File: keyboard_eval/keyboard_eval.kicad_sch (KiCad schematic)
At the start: 65 parts, among them IC1 IS31FL3733B-TQLS4, J1 Conn_01x03, J2 Conn_01x04, J3 Conn_01x04, J4 Conn_01x07, J5 Conn_01x03, J6 Conn_01x03, J7 Conn_01x06, SW1 RotaryEncoder_Switch

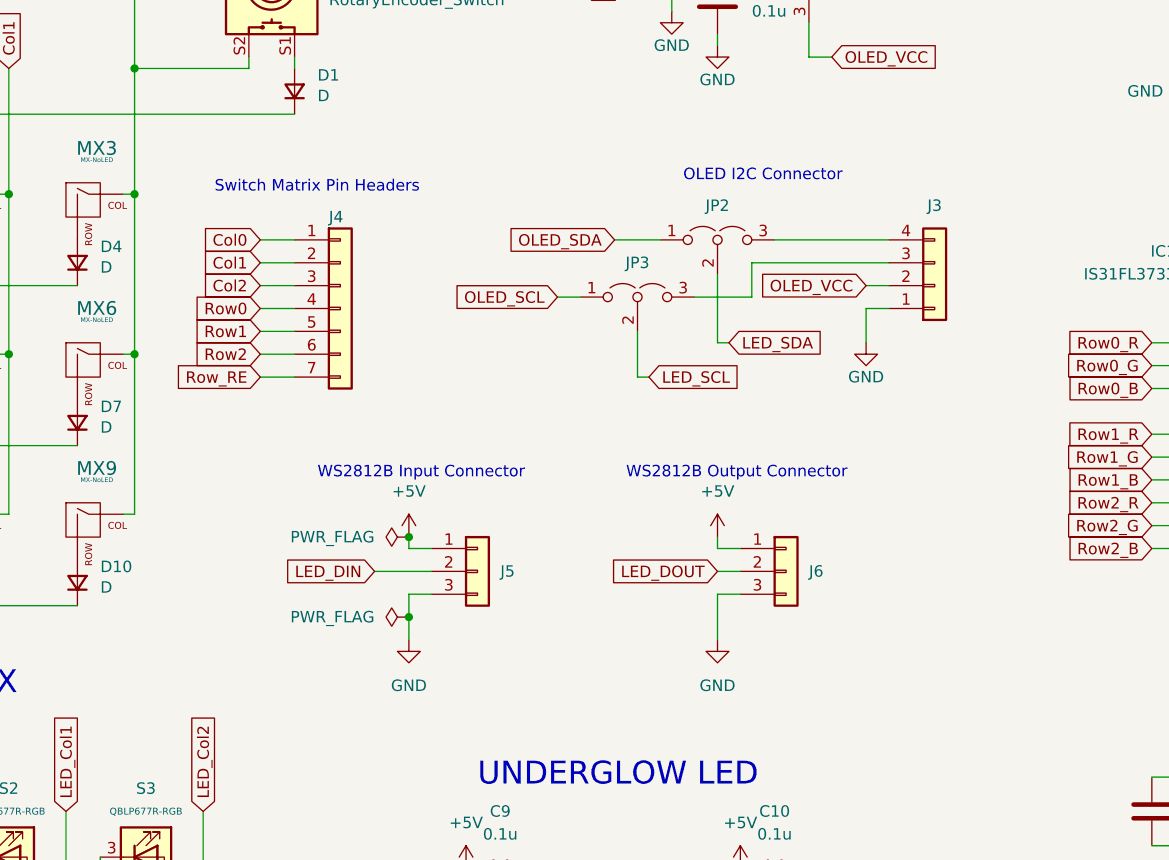
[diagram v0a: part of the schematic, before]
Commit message: WIP layout
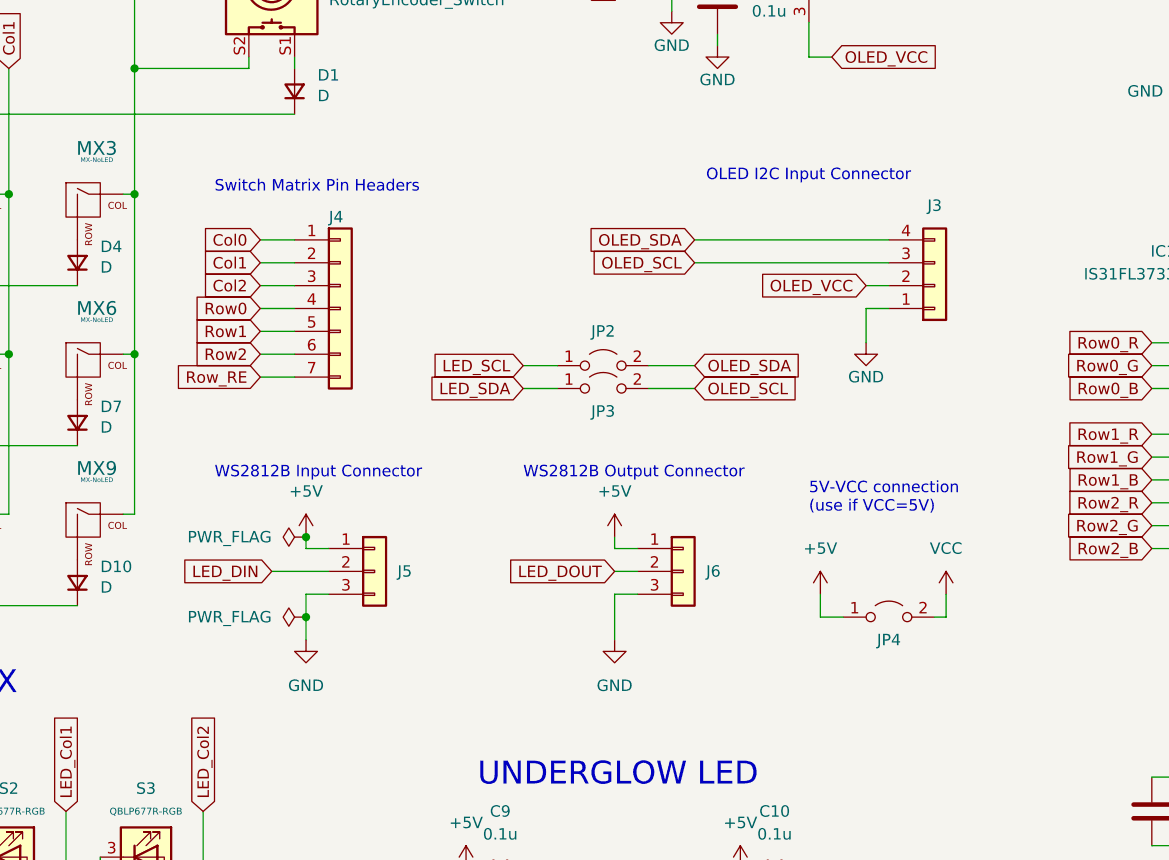
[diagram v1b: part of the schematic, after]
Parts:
- removed JP2, JP3: Jumper_3_Open, Jumper:SolderJumper-3_P1.3mm_Open_RoundedPad1.0x1.5mm, symbol Jumper:Jumper_3_Open
- added JP2, JP3, JP4: Jumper_2_Open, Jumper:SolderJumper-2_P1.3mm_Open_RoundedPad1.0x1.5mm, symbol Jumper:Jumper_2_Open
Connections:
- net +5V: now also JP4.1 (A)
- net LED_SCL: now also JP2.1 (A)
- net LED_SDA: now also JP3.1 (A)
- net OLED_SCL: now also J3.3 (Pin_3), JP3.2 (B)
- net OLED_SDA: now also J3.4 (Pin_4), JP2.2 (B)
- net VCC: now also JP4.2 (B)
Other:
- note added: "5V-VCC connection (use if VCC=5V)"
- note added: "OLED I2C Input Connector"
- note removed: "OLED I2C Connector"
- moved on the sheet: J5, J6
